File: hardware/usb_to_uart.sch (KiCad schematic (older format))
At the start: 13 parts, among them Q1 SS9013_J3, Q2 SS9013_J3, U7 CH340T, U8 USB_Micro, Y1 O_12M,3225

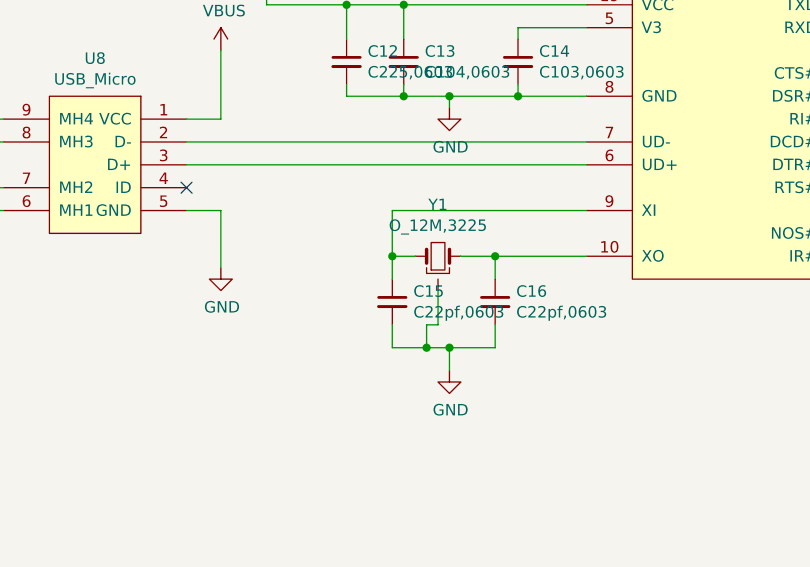
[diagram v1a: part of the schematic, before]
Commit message: update,
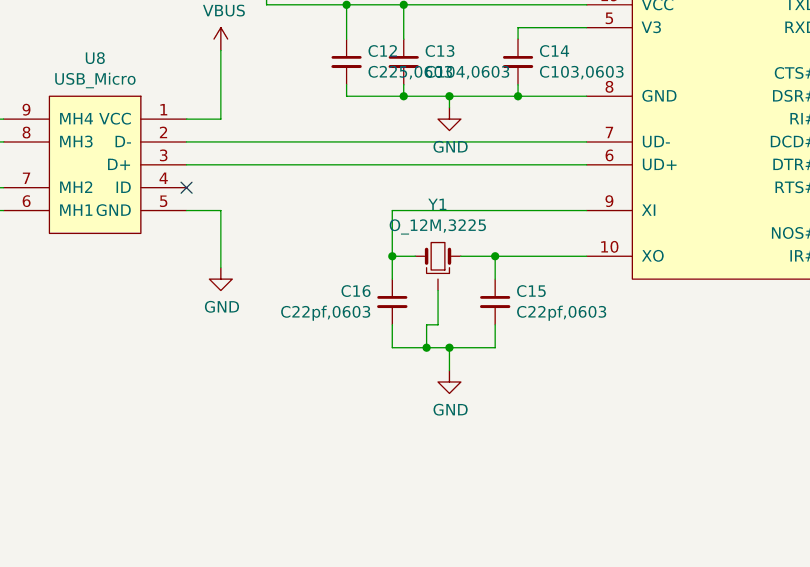
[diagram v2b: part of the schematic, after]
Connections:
- net at C16.1, Y1.3: now also U7.9 (XI); no longer U7.10 (XO)
- net at C15.1, Y1.1: now also U7.10 (XO); no longer U7.9 (XI)
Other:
- moved on the sheet: C15, C16
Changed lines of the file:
@@
 F 3 "~" H 3600 2700 50  0001 C CNN
 	1    3600 2700
-	1    0    0    -1
+	-1   0    0    -1
 $EndComp
 Wire Wire Line
@@
 L taobao-c:C22pf,0603 C15
 U 1 1 5D061A62
-P 3400 2900
-F 0 "C15" H 3492 2946 50  0000 L CNN
-F 1 "C22pf,0603" H 3492 2855 50  0000 L CNN
-F 2 "Capacitor_SMD:C_0603_1608Metric_Pad1.05x0.95mm_HandSolder" H 3400 2900 50  0001 C CNN
-F 3 "~" H 3400 2900 50  0001 C CNN
-	1    3400 2900
-	1    0    0    -1
-$EndComp
-$Comp
-L taobao-c:C22pf,0603 C16
-U 1 1 5D06326C
 P 3850 2900
-F 0 "C16" H 3942 2946 50  0000 L CNN
+F 0 "C15" H 3942 2946 50  0000 L CNN
 F 1 "C22pf,0603" H 3942 2855 50  0000 L CNN
 F 2 "Capacitor_SMD:C_0603_1608Metric_Pad1.05x0.95mm_HandSolder" H 3850 2900 50  0001 C CNN
@@
 	1    0    0    -1
 $EndComp
+$Comp
+L taobao-c:C22pf,0603 C16
+U 1 1 5D06326C
+P 3400 2900
+F 0 "C16" H 3309 2946 50  0000 R CNN
+F 1 "C22pf,0603" H 3309 2855 50  0000 R CNN
+F 2 "Capacitor_SMD:C_0603_1608Metric_Pad1.05x0.95mm_HandSolder" H 3400 2900 50  0001 C CNN
+F 3 "~" H 3400 2900 50  0001 C CNN
+	1    3400 2900
+	1    0    0    -1
+$EndComp
